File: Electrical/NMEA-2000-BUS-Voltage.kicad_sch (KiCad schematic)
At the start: 68 parts, among them IC1 ADS131M08QPBSRQ1, J1 DE9_Receptacle, J2 Conn_01x04, J3 Conn_01x02, J4 Conn_01x04, J5 Conn_01x05, J6 Conn_01x02, Q1 IRFZ44N, SW1 SW_Push, U1 ESP32-WROOM-32E, U2 LM7805_TO220, U3 AP2112K-3.3, U4 BME280, U5 SN65HVD230, U6 ADR4533, Y1 Crystal

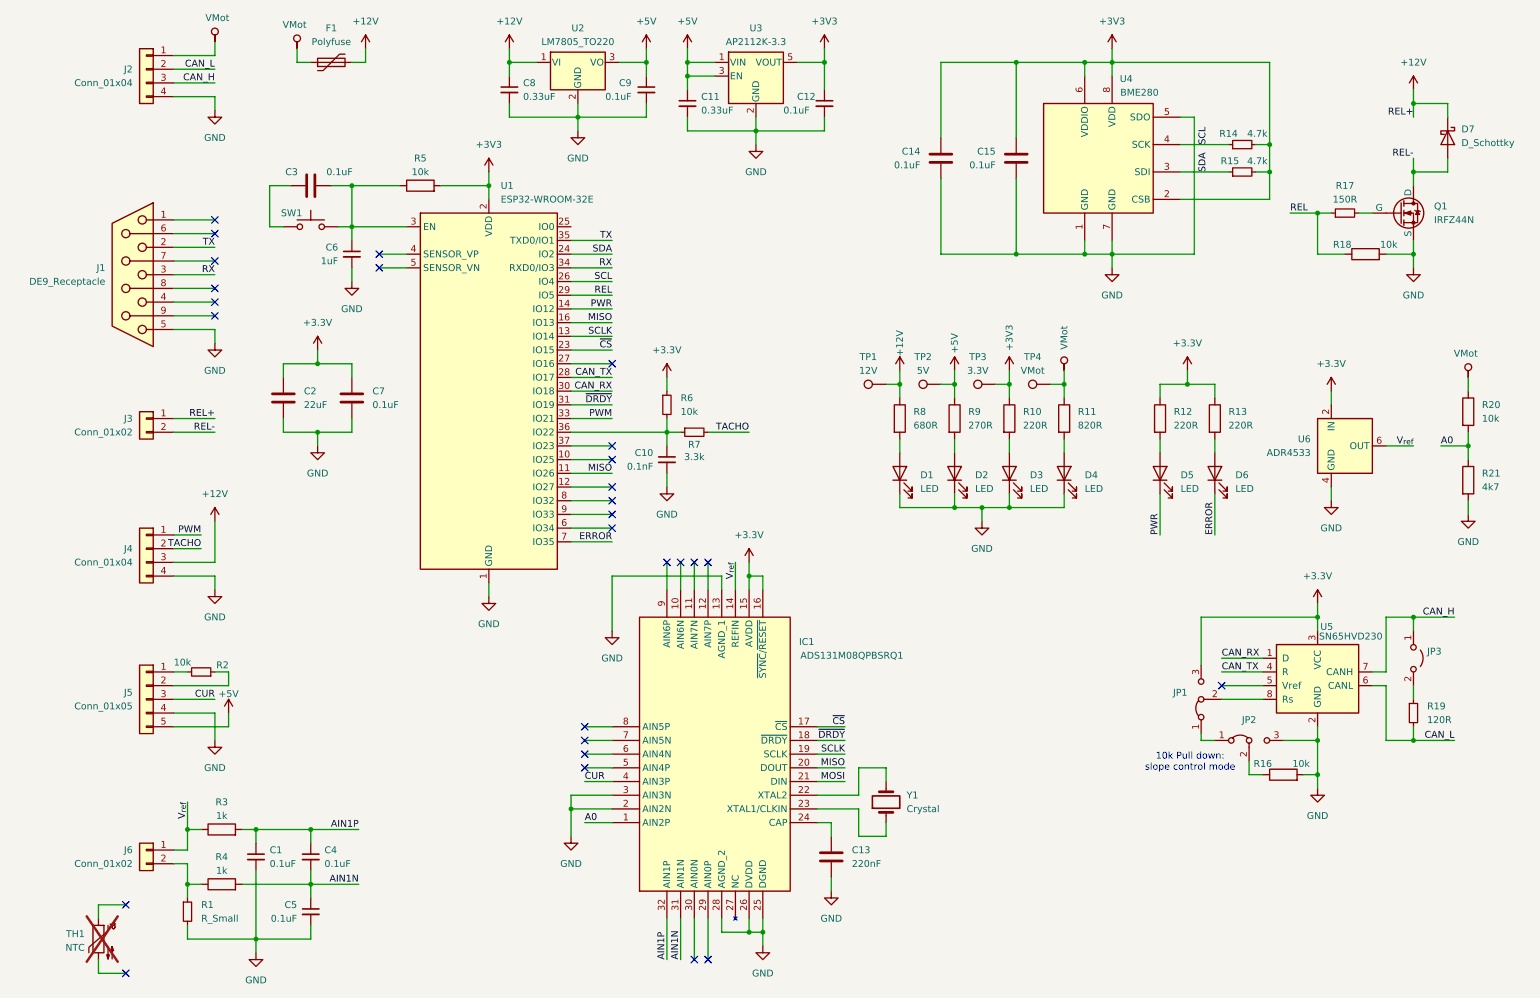
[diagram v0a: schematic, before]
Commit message: Updated Schematics
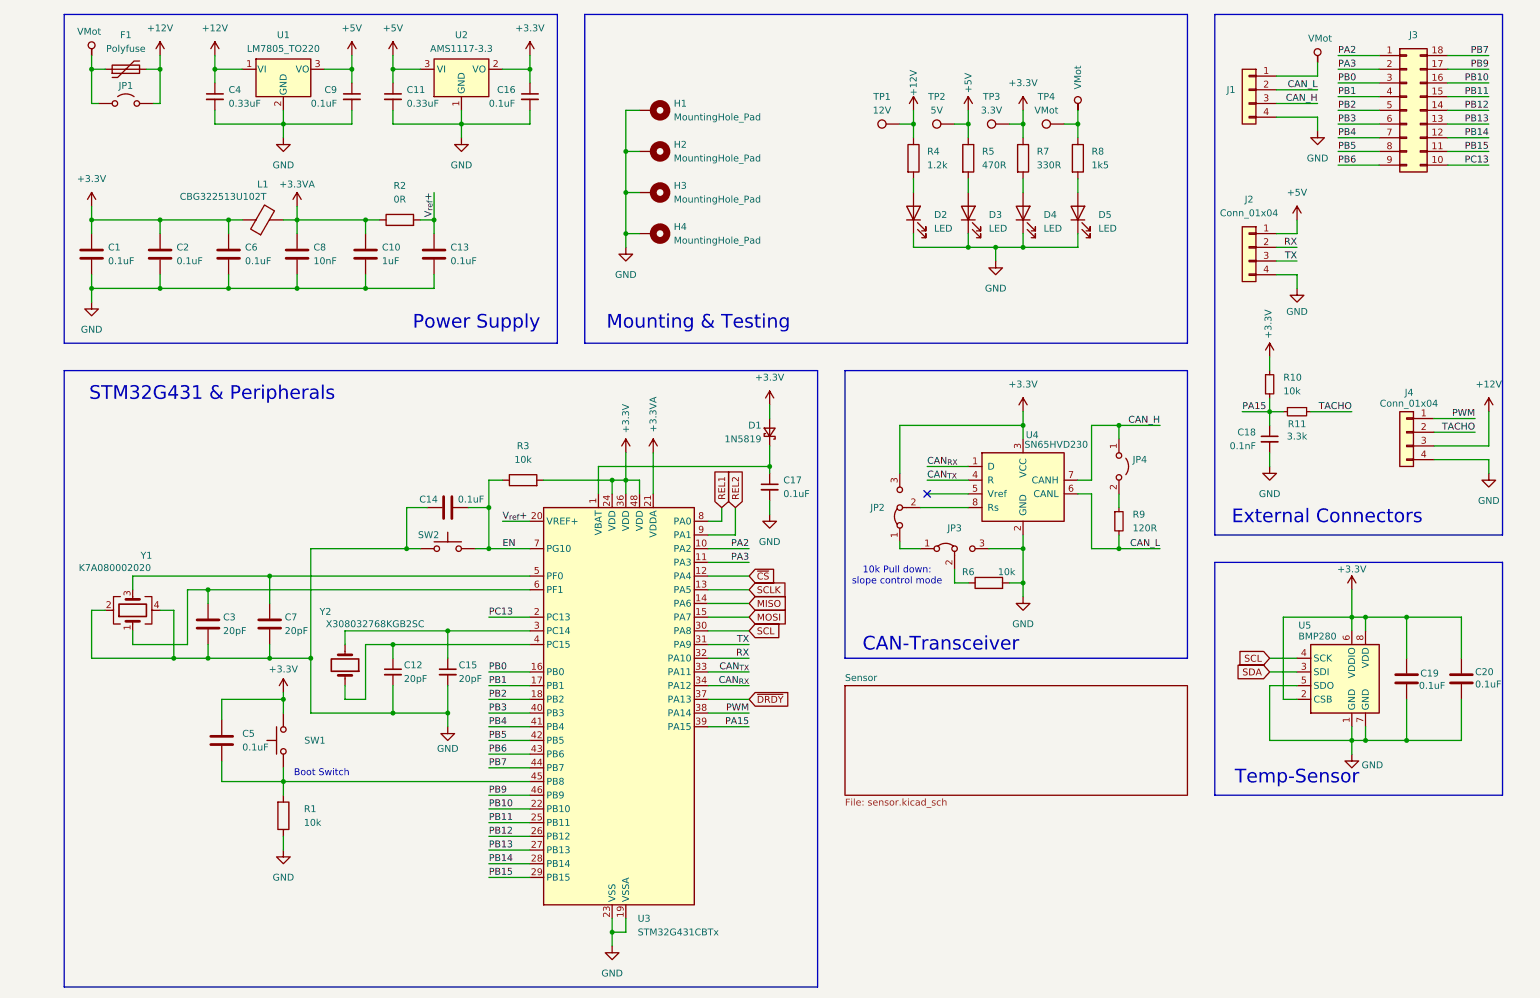
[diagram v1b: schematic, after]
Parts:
- removed C1, C4, C5: 0.1uF, Capacitor_THT:C_Disc_D3.0mm_W1.6mm_P2.50mm, symbol Device:C_Small
- removed C10: 0.1nF, Connector_PinHeader_2.54mm:PinHeader_1x02_P2.54mm_Vertical, symbol Device:C_Small
- removed C15: 0.1uF, Capacitor_THT:C_Disc_D3.0mm_W1.6mm_P2.50mm, symbol Device:C
- removed C6: 1uF, Capacitor_THT:C_Disc_D3.0mm_W1.6mm_P2.50mm, symbol Device:C_Small
- removed D5, D6: LED, LED_THT:LED_D5.0mm, symbol Device:LED
- removed D7: D_Schottky, Diode_THT:D_DO-201_P15.24mm_Horizontal, symbol Device:D_Schottky
- removed IC1: ADS131M08QPBSRQ1, symbol ADS131M08QPBSRQ1:ADS131M08QPBSRQ1
- removed J1: DE9_Receptacle, symbol Connector:DE9_Receptacle
- removed J3: Conn_01x02, TerminalBlock_Phoenix:TerminalBlock_Phoenix_PT-1,5-2-5.0-H_1x02_P5.00mm_Horizontal, symbol Connector_Generic:Conn_01x02
- removed J5: Conn_01x05, TerminalBlock_Phoenix:TerminalBlock_Phoenix_PT-1,5-5-5.0-H_1x05_P5.00mm_Horizontal, symbol Connector_Generic:Conn_01x05
- removed J6: Conn_01x02, symbol Connector_Generic:Conn_01x02
- removed Q1: IRFZ44N, Package_TO_SOT_THT:TO-220-3_Vertical, symbol Simulation_SPICE:NMOS
- removed R1: R_Small, symbol Device:R_Small
- removed R12, R13: 220R, symbol Device:R
- removed R14, R15: 4.7k, symbol Device:R_Small
- removed R17: 150R, symbol Device:R_Small
- removed R18, R5: 10k, symbol Device:R
- removed R2, R6: 10k, Resistor_THT:R_Axial_DIN0204_L3.6mm_D1.6mm_P5.08mm_Horizontal, symbol Device:R_Small
- removed R20: 10k, Resistor_THT:R_Axial_DIN0204_L3.6mm_D1.6mm_P5.08mm_Horizontal, symbol Device:R
- removed R21: 4k7, Resistor_THT:R_Axial_DIN0204_L3.6mm_D1.6mm_P5.08mm_Horizontal, symbol Device:R
- removed R4: 1k, symbol Device:R
- removed R7: 3.3k, Resistor_THT:R_Axial_DIN0204_L3.6mm_D1.6mm_P5.08mm_Horizontal, symbol Device:R_Small
- removed TH1: NTC, symbol Device:Thermistor_NTC
- removed U1: ESP32-WROOM-32E, RF_Module:ESP32-WROOM-32D, symbol RF_Module:ESP32-WROOM-32E
- removed U3: AP2112K-3.3, Package_TO_SOT_SMD:SOT-23-5, symbol Regulator_Linear:AP2112K-3.3
- removed U4: BME280, Package_LGA:Bosch_LGA-8_2.5x2.5mm_P0.65mm_ClockwisePinNumbering, symbol Sensor:BME280
- removed U6: ADR4533, Package_SO:SOIC-8_3.9x4.9mm_P1.27mm, symbol Reference_Voltage:ADR4533
- removed Y1: Crystal, symbol Device:Crystal
- added C1, C19, C20, C5, C6: 0.1uF, Capacitor_THT:C_Disc_D5.0mm_W2.5mm_P5.00mm, symbol Device:C
- added C10: 1uF, Capacitor_THT:C_Disc_D5.0mm_W2.5mm_P5.00mm, symbol Device:C
- added C12, C15: 20pF, Capacitor_THT:C_Disc_D5.0mm_W2.5mm_P5.00mm, symbol Device:C_Small
- added C17: 0.1uF, Capacitor_THT:C_Disc_D5.0mm_W2.5mm_P5.00mm, symbol Device:C_Small
- added C18: 0.1nF, Capacitor_THT:C_Disc_D5.0mm_W2.5mm_P5.00mm, symbol Device:C_Small
- added C8: 10nF, Capacitor_THT:C_Disc_D5.0mm_W2.5mm_P5.00mm, symbol Device:C
- added D1: 1N5819, Diode_THT:D_DO-41_SOD81_P10.16mm_Horizontal, symbol Device:D_Schottky_Small
- added H1, H2, H3, H4: MountingHole_Pad, MountingHole:MountingHole_6mm_Pad, symbol Mechanical:MountingHole_Pad
- added J2: Conn_01x04, Connector_PinSocket_2.54mm:PinSocket_1x04_P2.54mm_Horizontal, symbol Connector_Generic:Conn_01x04
- added J3: Conn_02x08_Counter_Clockwise, Connector_PinHeader_2.54mm:PinHeader_2x09_P2.54mm_Vertical, symbol Connector_Generic:Conn_02x09_Counter_Clockwise
- added JP1: Jumper_2_Open, Connector_PinHeader_2.54mm:PinHeader_1x02_P2.54mm_Vertical, symbol Jumper:Jumper_2_Open
- added L1: CBG322513U102T, Inductor_SMD:L_1210_3225Metric_Pad1.42x2.65mm_HandSolder, symbol Device:FerriteBead
- added R1: 10k, Resistor_THT:R_Axial_DIN0207_L6.3mm_D2.5mm_P10.16mm_Horizontal, symbol Device:R
- added R10: 10k, Resistor_THT:R_Axial_DIN0207_L6.3mm_D2.5mm_P10.16mm_Horizontal, symbol Device:R_Small
- added R11: 3.3k, Resistor_THT:R_Axial_DIN0207_L6.3mm_D2.5mm_P10.16mm_Horizontal, symbol Device:R_Small
- added R2: 0R, Resistor_THT:R_Axial_DIN0207_L6.3mm_D2.5mm_P10.16mm_Horizontal, symbol Device:R
- added SW2: SW_Push, Button_Switch_THT:SW_PUSH_6mm, symbol Switch:SW_Push
- added U2: AMS1117-3.3, Package_TO_SOT_SMD:SOT-223-3_TabPin2, symbol Regulator_Linear:AMS1117-3.3
- added U3: STM32G431CBTx, Package_QFP:LQFP-48_7x7mm_P0.5mm, symbol MCU_ST_STM32G4:STM32G431CBTx
- added U5: BMP280, N2K-influx:Bosch_LGA-8_2x2.5mm_P0.65mm_ClockwisePinNumbering, symbol Sensor_Pressure:BMP280
- added Y1: K7A080002020, Crystal:Crystal_SMD_7050-4Pin_7.0x5.0mm, symbol Device:Crystal_GND24
- added Y2: X308032768KGB2SC, Crystal:Crystal_C38-LF_D3.0mm_L8.0mm_Horizontal, symbol Device:Crystal
- C11, C14, C9: footprint Capacitor_THT:C_Disc_D3.0mm_W1.6mm_P2.50mm -> Capacitor_THT:C_Disc_D5.0mm_W2.5mm_P5.00mm
- C13: value 220nF -> 0.1uF; footprint Capacitor_THT:C_Disc_D3.0mm_W1.6mm_P2.50mm -> Capacitor_THT:C_Disc_D5.0mm_W2.5mm_P5.00mm
- C16: renamed from C12; footprint Capacitor_THT:C_Disc_D3.0mm_W1.6mm_P2.50mm -> Capacitor_THT:C_Disc_D5.0mm_W2.5mm_P5.00mm
- C2: value 22uF -> 0.1uF; footprint Capacitor_THT:C_Disc_D3.0mm_W1.6mm_P2.50mm -> Capacitor_THT:C_Disc_D5.0mm_W2.5mm_P5.00mm
- C3, C7: value 0.1uF -> 20pF; footprint Capacitor_THT:C_Disc_D3.0mm_W1.6mm_P2.50mm -> Capacitor_THT:C_Disc_D5.0mm_W2.5mm_P5.00mm
- C4: renamed from C8; footprint Capacitor_THT:C_Disc_D3.0mm_W1.6mm_P2.50mm -> Capacitor_THT:C_Disc_D5.0mm_W2.5mm_P5.00mm
- F1: footprint Diode_THT:D_DO-247_Horizontal_TabDown -> Diode_SMD:D_1210_3225Metric_Pad1.42x2.65mm_HandSolder
- JP2: renamed from JP1; footprint Connector_PinSocket_2.54mm:PinSocket_1x03_P2.54mm_Vertical -> Connector_PinHeader_2.54mm:PinHeader_1x03_P2.54mm_Vertical
- JP3: renamed from JP2; footprint Connector_PinSocket_2.54mm:PinSocket_1x03_P2.54mm_Vertical -> Connector_PinHeader_2.54mm:PinHeader_1x03_P2.54mm_Vertical
- R3: value 1k -> 10k; footprint (none) -> Resistor_THT:R_Axial_DIN0207_L6.3mm_D2.5mm_P10.16mm_Horizontal
- R4: renamed from R8; value 680R -> 1.2k; footprint Resistor_THT:R_Axial_DIN0204_L3.6mm_D1.6mm_P5.08mm_Horizontal -> Resistor_THT:R_Axial_DIN0207_L6.3mm_D2.5mm_P10.16mm_Horizontal
- R5: renamed from R9; value 270R -> 470R; footprint Resistor_THT:R_Axial_DIN0204_L3.6mm_D1.6mm_P5.08mm_Horizontal -> Resistor_THT:R_Axial_DIN0207_L6.3mm_D2.5mm_P10.16mm_Horizontal
- R6: renamed from R16; footprint (none) -> Resistor_THT:R_Axial_DIN0207_L6.3mm_D2.5mm_P10.16mm_Horizontal
- R7: renamed from R10; value 220R -> 330R; footprint Resistor_THT:R_Axial_DIN0204_L3.6mm_D1.6mm_P5.08mm_Horizontal -> Resistor_THT:R_Axial_DIN0207_L6.3mm_D2.5mm_P10.16mm_Horizontal
- R8: renamed from R11; value 820R -> 1k5; footprint Resistor_THT:R_Axial_DIN0204_L3.6mm_D1.6mm_P5.08mm_Horizontal -> Resistor_THT:R_Axial_DIN0207_L6.3mm_D2.5mm_P10.16mm_Horizontal
- R9: renamed from R19; footprint Resistor_THT:R_Axial_DIN0204_L3.6mm_D1.6mm_P5.08mm_Horizontal -> Resistor_THT:R_Axial_DIN0207_L6.3mm_D2.5mm_P10.16mm_Horizontal
- SW1: footprint (none) -> Button_Switch_THT:SW_PUSH_6mm
- TP1, TP2, TP3, TP4: footprint (none) -> TestPoint:TestPoint_Pad_3.0x3.0mm
- renumbered D1 to D2, D2 to D3, D3 to D4, D4 to D5, J2 to J1, JP3 to JP4, U2 to U1, U5 to U4
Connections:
- net AIN1P is gone; now on net +3.3V: R3.2
- net +12V: now also JP1.2 (B)
- net +3.3V: now also C16.1, R7.1, SW1.1, TP3.1, C1.1, C19.1, C20.1, C5.1, C6.1, D1.2 (A), L1.1, R10.1, U2.2 (VO), U3.24 (VDD), U3.36 (VDD), U3.48 (VDD), U5.2 (CSB), U5.6 (VDDIO), U5.8 (VDD); no longer C7.1
- net +5V: now also J2.1 (Pin_1), U2.3 (VI)
- net GND: now also C14.1, C3.2, C1.2, C10.2, C12.2, C15.2, C17.2, C18.2, C19.2, C20.2, C6.2, C8.2, H1.1, H2.1, H3.1, H4.1, J2.4 (Pin_4), R1.1, SW2.1, U2.1 (GND), U3.19 (VSSA), U3.23 (VSS), U3.35 (VSS), U3.47 (VSS), U5.1 (GND), U5.5 (SDO), U5.7 (GND), Y1.2, Y1.4; no longer C14.2
- net MISO: now also U3.14 (PA6)
- net MOSI: now also U3.15 (PA7)
- net PWM: now also U3.38 (PA14)
- net RX: now also J2.2 (Pin_2), U3.32 (PA10)
- net SCL: now also U3.30 (PA8), U5.4 (SCK)
- net SCLK: now also U3.13 (PA5)
- net SDA: now also U5.3 (SDI)
- net TACHO: now also R11.2
- net TX: now also J2.3 (Pin_3), U3.31 (PA9)
- net VMot: now also JP1.1 (A)
- net ~{CS}: now also U3.12 (PA4)
- net ~{DRDY}: now also U3.37 (PA13)
- net at SW1.2: now also C5.2, R1.2, U3.45 (PB8); no longer C3.2
- net V_{ref}+: now reaches C13.1
- net V_{ref}+: now also R2.2, U3.20 (VREF+)
- net at C3.1: now also U3.6 (PF1), Y1.1; no longer SW1.1
- removed net +3V3: C14.1, C16.1, R7.1, TP3.1
- net CAN_RX renamed CAN_{RX}
- net CAN_{RX}: now also U3.34 (PA12)
- net CAN_TX renamed CAN_{TX}
- net CAN_{TX}: now also U3.33 (PA11)
- net V_{ref} renamed EN
- net EN: now also C14.2, SW2.2, U3.7 (PG10)
- new net: C17.1, D1.1 (K), U3.1 (VBAT)
- new net: C7.1, U3.5 (PF0), Y1.3
- new net: C12.1, U3.4 (PC15), Y2.1
- new net: C15.1, U3.3 (PC14), Y2.2
- new net +3.3VA: C10.1, C8.1, L1.2, R2.1, U3.21 (VDDA)
- new net PA15: C18.1, R10.2, R11.1, U3.39 (PA15)
- new net PA2: J3.1 (Pin_1), U3.10 (PA2)
- new net PA3: J3.2 (Pin_2), U3.11 (PA3)
- new net PB0: J3.3 (Pin_3), U3.16 (PB0)
- new net PB1: J3.4 (Pin_4), U3.17 (PB1)
- new net PB10: J3.16 (Pin_16), U3.22 (PB10)
- new net PB11: J3.15 (Pin_15), U3.25 (PB11)
- new net PB12: J3.14 (Pin_14), U3.26 (PB12)
- new net PB13: J3.13 (Pin_13), U3.27 (PB13)
- new net PB14: J3.12 (Pin_12), U3.28 (PB14)
- new net PB15: J3.11 (Pin_11), U3.29 (PB15)
- new net PB2: J3.5 (Pin_5), U3.18 (PB2)
- new net PB3: J3.6 (Pin_6), U3.40 (PB3)
- new net PB4: J3.7 (Pin_7), U3.41 (PB4)
- new net PB5: J3.8 (Pin_8), U3.42 (PB5)
- new net PB6: J3.9 (Pin_9), U3.43 (PB6)
- new net PB7: J3.18 (Pin_18), U3.44 (PB7)
- new net PB9: J3.17 (Pin_17), U3.46 (PB9)
- new net PC13: J3.10 (Pin_10), U3.2 (PC13)
- new net REL1: U3.8 (PA0)
- new net REL2: U3.9 (PA1)
- no-connect marks 28 -> 1
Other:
- added sheet Sensor (sensor.kicad_sch)
- note added: "Boot Switch"
- note added: "CAN-Transceiver"
- note added: "External Connectors"
- note added: "Mounting & Testing"
- note added: "Power Supply"
- note added: "STM32G431 & Peripherals"
- note added: "Temp-Sensor"
- moved on the sheet: C11, C16, C4, C9, D2, D3, D4, D5, F1, J1, J4, JP2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
